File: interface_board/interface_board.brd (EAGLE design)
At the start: 65 x 56 mm, 93 parts, among them IC1 V7805-1000, IC6 LAN9512-JZX, K2 61400826021, Q1 IRLML6346TRPBF, Q6 FA-238 25.0000MB, U1 AL5812MP-13, U2 MPU-9250

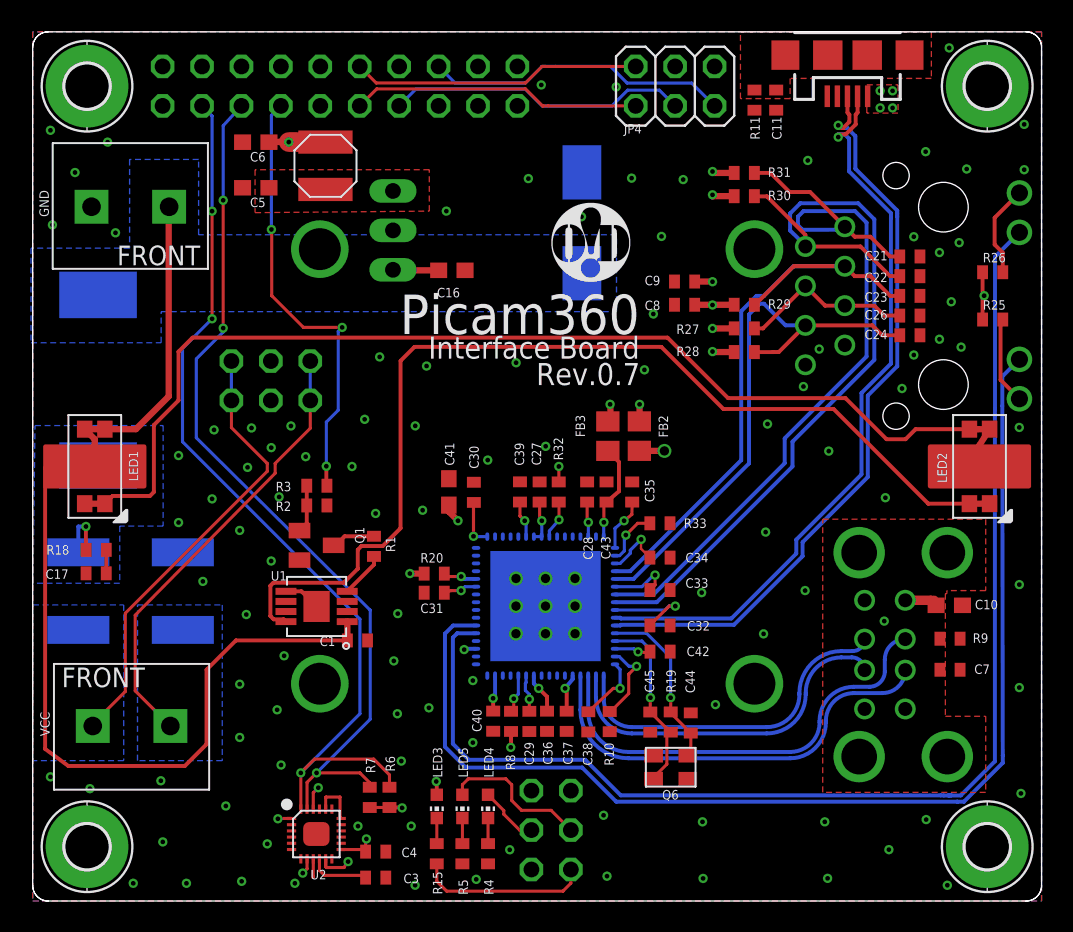
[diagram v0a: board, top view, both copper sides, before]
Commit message: interface board
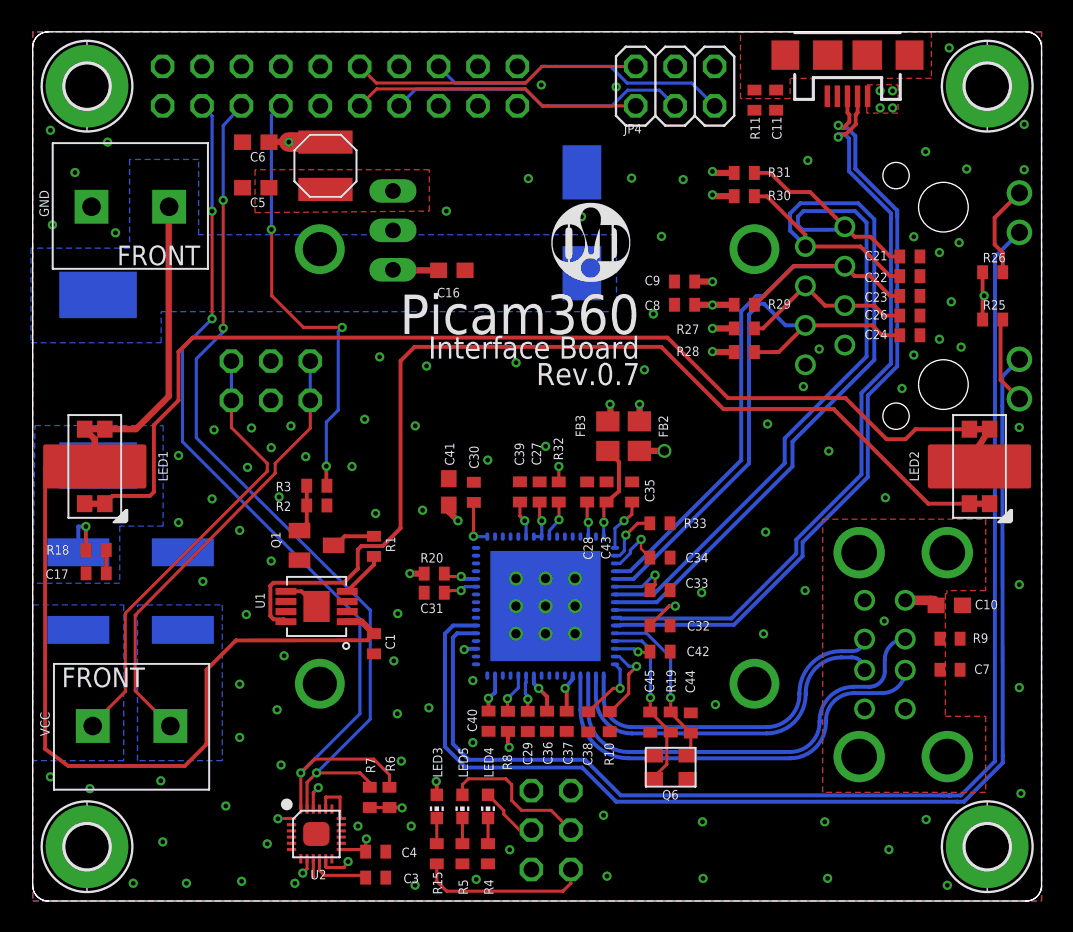
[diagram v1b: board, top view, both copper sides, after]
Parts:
- moved C1 1.09 mm to (22.0, 16.6), turned to 90 degrees
- moved C40 0.30 mm to (29.4, 11.6)
- moved R8 0.20 mm to (30.6, 11.6)
- moved C29 0.10 mm to (31.9, 11.6)
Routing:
- net +12V: track 72.7 -> 75.5 mm

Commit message: revert to 2.7mm hole for camera
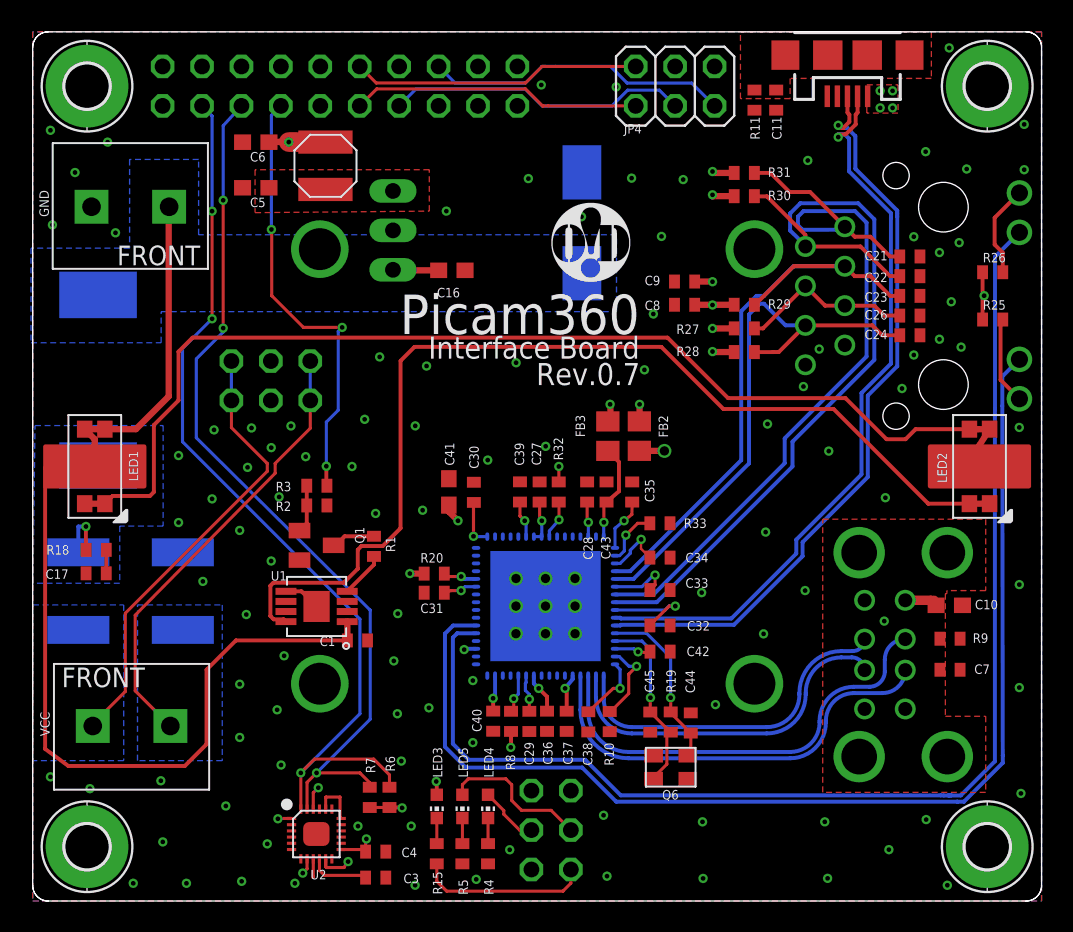
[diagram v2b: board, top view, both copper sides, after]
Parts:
- moved C1 1.09 mm to (20.9, 16.8), turned to 180 degrees
- moved C40 0.30 mm to (29.7, 11.6)
- moved R8 0.20 mm to (30.8, 11.6)
- moved C29 0.10 mm to (32.0, 11.6)
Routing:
- net +12V: track 75.5 -> 72.7 mm
